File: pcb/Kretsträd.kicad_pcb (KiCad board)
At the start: 2 copper layers, 112.2 x 95.8 mm, 52 parts, among them J1 Conn_01x02_Female, J2 Conn_01x02_Female, J3 Conn_01x02_Female, J4 Conn_01x02_Female, SW1 SW_PUSH, SW10 SW_PUSH, SW11 SW_PUSH, SW12 SW_PUSH, SW13 SW_PUSH, SW14 SW_PUSH, SW15 SW_PUSH, SW16 SW_PUSH, SW17 SW_PUSH, SW2 SW_PUSH, SW3 SW_PUSH, SW4 SW_PUSH, SW5 SW_PUSH, SW6 SW_PUSH, SW7 SW_PUSH, SW8 SW_PUSH, SW9 SW_PUSH, U1 SeeeduinoXIAO

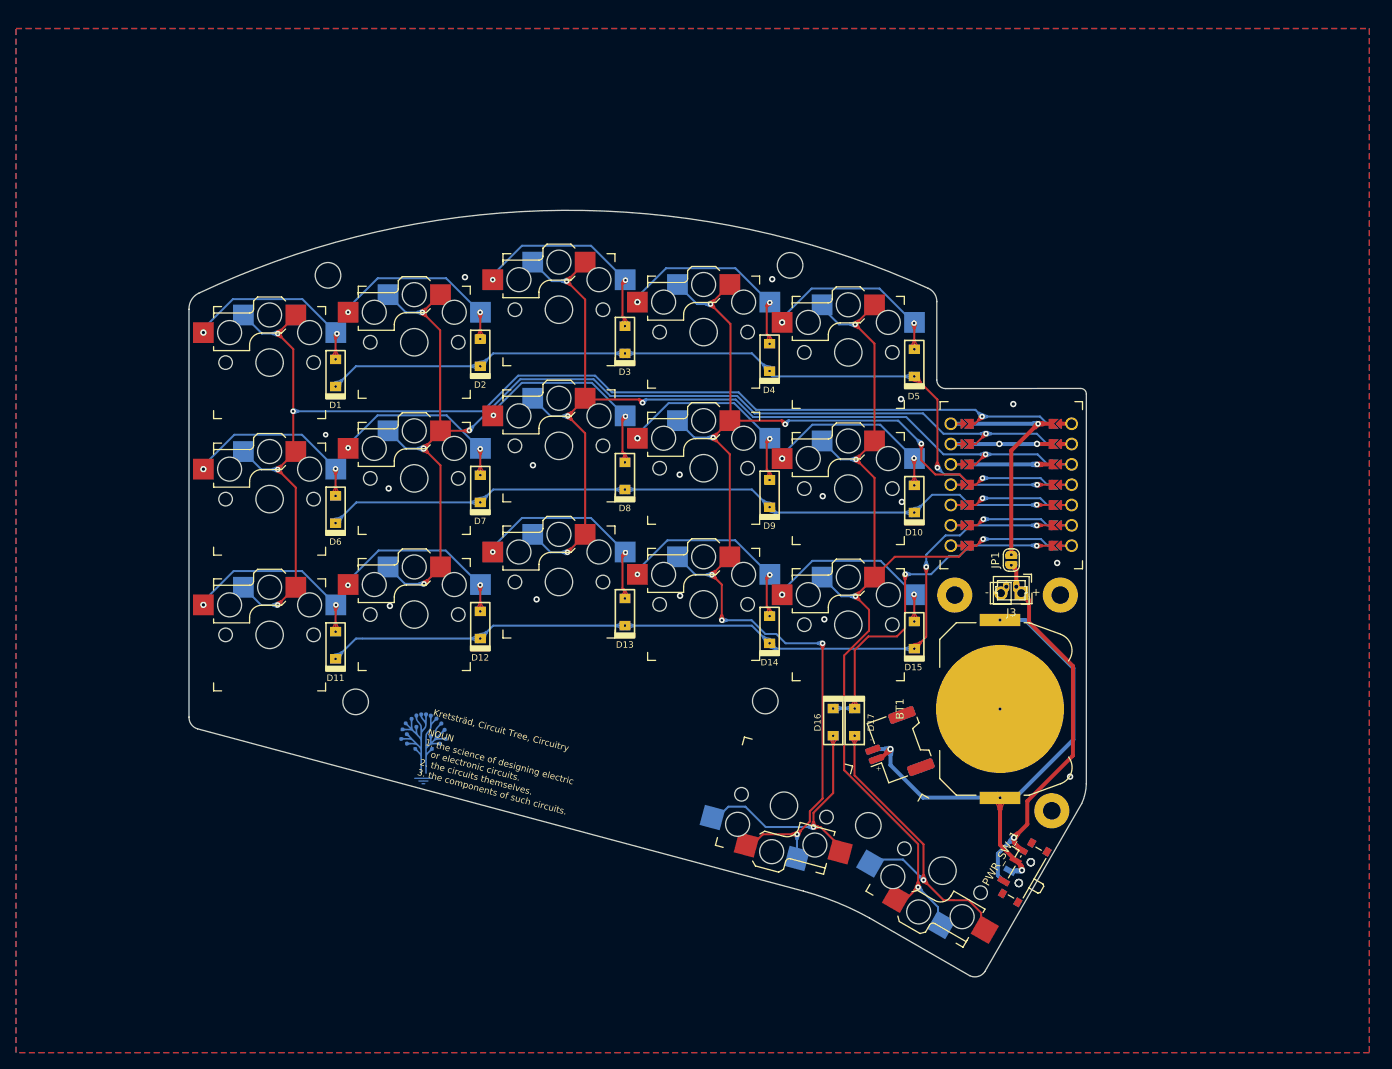
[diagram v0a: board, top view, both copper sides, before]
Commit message: First public version.
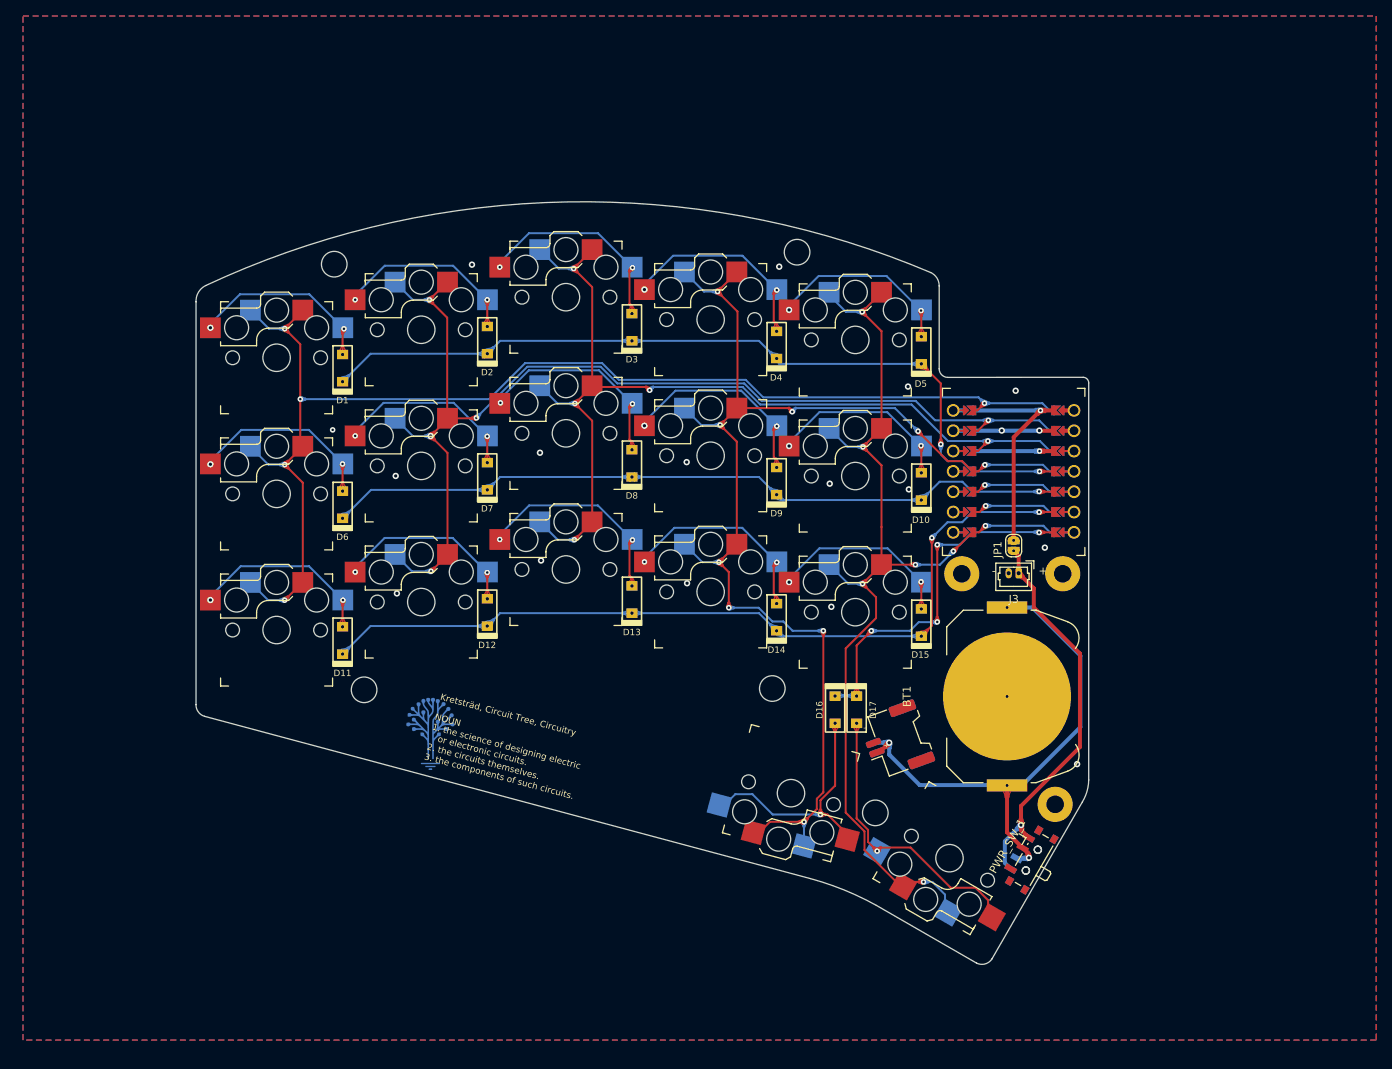
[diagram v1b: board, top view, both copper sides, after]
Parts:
- removed J4: Conn_01x02_Female, Connector_PinSocket_2.54mm:PinSocket_1x02_P2.54mm_Vertical
- moved TH_PCB_1 2.80 mm to (176.0, 93.0)
- moved TH_PCB_2 2.68 mm to (188.6, 93.0)
- moved G*** 2.02 mm to (109.3, 111.9)
- moved TH2 1.87 mm to (155.4, 52.8)
- moved TH3 1.84 mm to (101.2, 107.5)
- moved JP1 1.83 mm to (182.4, 89.4)
- moved D14 1.79 mm to (152.8, 98.4)
- moved D4 1.79 mm to (152.8, 64.4)
- moved D9 1.79 mm to (152.8, 81.4)
- moved SW14 1.79 mm to (144.6, 95.2)
- moved SW16 1.79 mm to (154.6, 120.4)
- moved SW9 1.79 mm to (144.6, 78.2)
- moved D3 1.79 mm to (134.7, 62.2)
- moved SW4 1.79 mm to (144.6, 61.2)
- moved SW5 1.79 mm to (162.6, 63.7)
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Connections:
- SW10 pad : (no net) -> col4
- SW14 pad : (no net) -> col3
- SW15 pad : (no net) -> col4
- SW16 pad : (no net) -> col3
- SW17 pad : (no net) -> col4
- SW4 pad : (no net) -> col3
- SW5 pad : (no net) -> col4
- SW9 pad : (no net) -> col3
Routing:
- net Net-(D17-Pad2): track 39.3 -> 35.4 mm
- net col3: track 154.2 -> 151.3 mm
- net /PWR: track 47.8 -> 49.3 mm
- net row3: track 43.9 -> 45.1 mm, vias 2 -> 4
- net col0: track 155.0 -> 154.4 mm
- net col2: track 118.2 -> 117.6 mm
- net col1: track 139.4 -> 138.8 mm
- net col4: vias 5 -> 7
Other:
- board size 112.2 x 95.8 mm -> 111.6 x 95.3 mm
